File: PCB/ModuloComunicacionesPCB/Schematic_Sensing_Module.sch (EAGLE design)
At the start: 63 parts, among them IC1 MCP3202P, Q1 CSM-7X-DU, SW2 1825910-6, U1 ATMEGA328P-PU, U2 LP38690DT-5.0, U2_VCC NCP699SN33T1G, U3_VDD NCP699SN33T1G

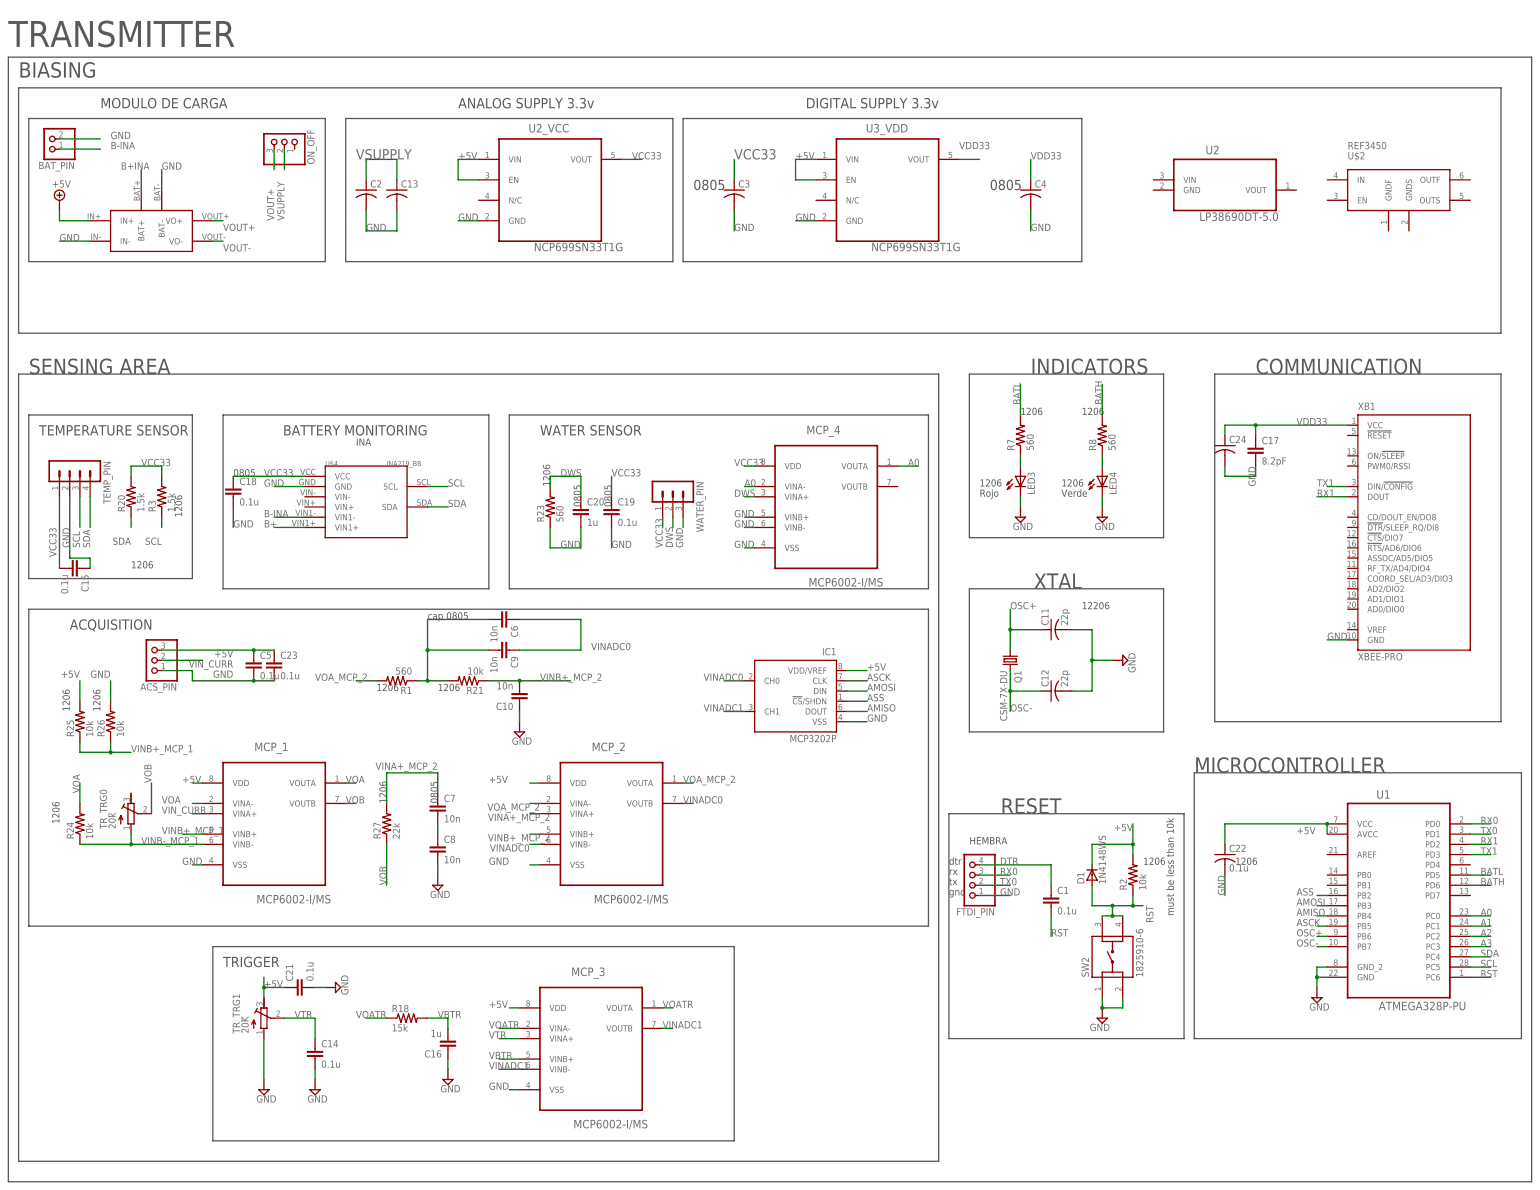
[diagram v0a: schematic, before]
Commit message: avance en esquematico para la PCB
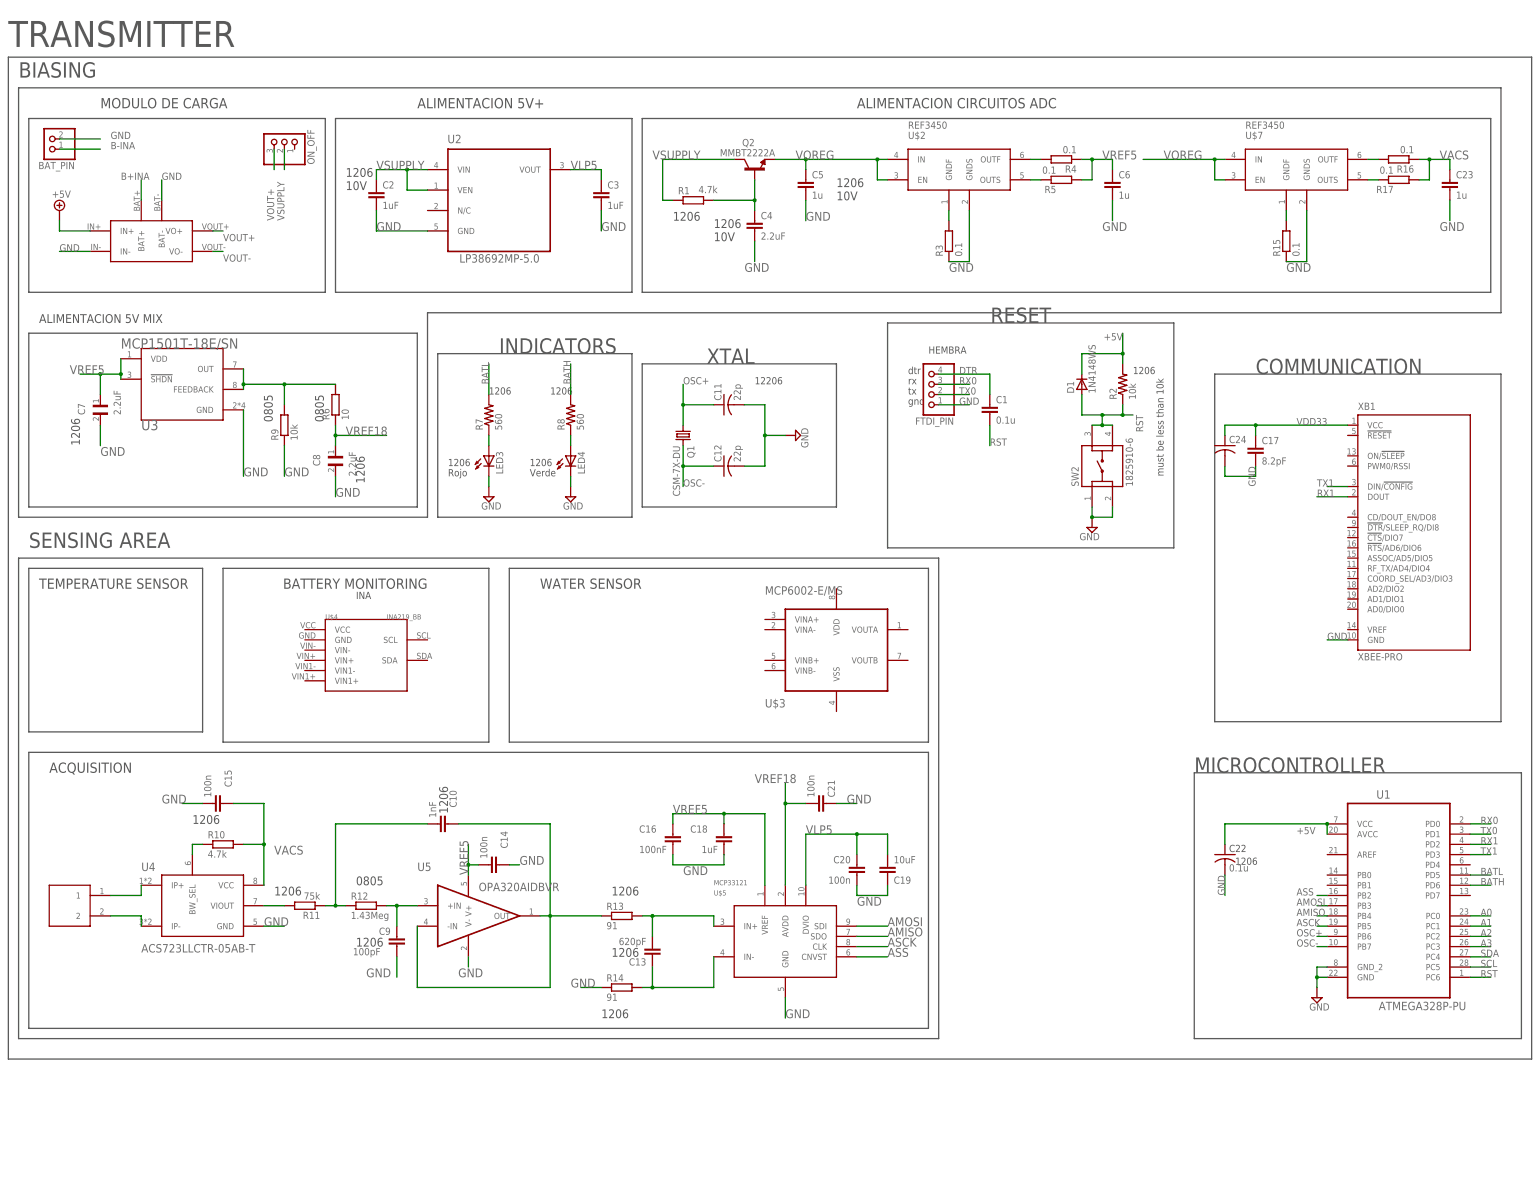
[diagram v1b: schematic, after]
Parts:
- removed ACS_PIN: (no value), pinhead:PINHD-1X3
- removed IC1: MCP3202P, microchip:MCP3202P
- removed MCP_1: MCP6002-I/MS, MCP6002-I_MS-2:MCP6002-I/MS
- removed MCP_2, MCP_3, MCP_4: MCP6002-I/MS, MCP6002-I_MS:MCP6002-I/MS
- removed R18: 15k, resistor:R-US_R0805
- removed R20: 1.5k, rcl:R-US_R1206
- removed R21, R24, R25, R26: 10k, rcl:R-US_R1206
- removed R23: 560, rcl:R-US_R1206
- removed R27: 22k, rcl:R-US_R1206
- removed TEMP_PIN: (no value), con-lstb:MA04-1
- removed TR_TRG0: 20k, rcl:R-TRIMM64W
- removed TR_TRG1: 20K, rcl:R-TRIMM64W
- removed U2_VCC, U3_VDD: NCP699SN33T1G, NCP699SN33T1G:NCP699SN33T1G
- removed WATER_PIN: (no value), con-lstb:MA03-1
- added Q2: MMBT2222A, MMBT2222A:MMBT2222A
- added R10: 4.7k, rcl:R-EU_M1206
- added R11: 75k, rcl:R-EU_R1206
- added R12: 1.43Meg, rcl:R-EU_R0805
- added R13, R14: 91, rcl:R-EU_R1206
- added R15, R16, R17, R4, R5: 0.1, rcl:R-EU_R1206
- added R6: 10, rcl:R-EU_R0805
- added R9: 10k, rcl:R-EU_R0805
- added U$3: MCP6002-E/MS, MCP6002-E_MS:MCP6002-E/MS
- added U$5: MCP33121, mcp33121:MCP33121
- added U$6: TERMINAL-TB2, TERMINAL-TB001:TERMINAL-TB2
- added U$7: REF3450, SOT95P280X145-6N:REF3450
- added U3: MCP1501T-18E/SN, MCP1501T-18E_SN:MCP1501T-18E/SN
- added U4: ACS723LLCTR-05AB-T, ACS723LLCTR-05AB-T:ACS723LLCTR-05AB-T
- added U5: OPA320AIDBVR, OPA320AIDBVR:OPA320AIDBVR
- C10: value 10n -> 1nF; device rcl:C-EUC0805 -> rcl:C-EUC1206
- C13: value (none) -> 620pF; device rcl:C-USC0805 -> rcl:C-EUC1206
- C14, C15, C21: value 0.1u -> 100n; device rcl:C-EUC0805 -> rcl:C-EUC1206
- C16: value 1u -> 100nF; device rcl:C-EUC0805 -> rcl:C-EUC1206
- C18: value 0.1u -> 1uF; device rcl:C-EUC0805 -> rcl:C-EUC1206
- C19: value 0.1u -> 10uF; device rcl:C-EUC0805 -> rcl:C-EUC1206
- C2, C3: value (none) -> 1uF; device rcl:C-USC0805 -> rcl:C-EUC1206
- C20: value 1u -> 100n; device rcl:C-EUC0805 -> rcl:C-EUC1206
- C23, C5: value 0.1u -> 1u; device rcl:C-EUC0805 -> rcl:C-EUC1206
- C4: value (none) -> 2.2uF; device rcl:C-USC0805 -> rcl:C-EUC1206
- C6: value 10n -> 1u; device rcl:C-EUC0805 -> rcl:C-EUC1206
- C7, C8: value 10n -> 2.2uF; device rcl:C-EUC0805 -> T491A106K010AT7280:T491A106K010AT7280
- C9: value 10n -> 100pF; device rcl:C-EUC0805 -> rcl:C-EUC1206
- R1: value 560 -> 4.7k; device rcl:R-US_R1206 -> rcl:R-EU_R1206
- R3: value 1.5k -> 0.1; device rcl:R-US_R1206 -> rcl:R-EU_R1206
- U2: value LP38690DT-5.0 -> LP38692MP-5.0; device LP38690DT-5.0:LP38690DT-5.0 -> LP38692MP-5.0:LP38692MP-5.0
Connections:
- removed net B+: U$4.VIN1+
- removed net DWS: C20.1, MCP_4.VINA+, R23.2, WATER_PIN.2
- removed net VBTR: C16.2, MCP_3.VINB+, R18.2
- removed net VCC33: C15.2, C18.1, C19.1, C3.1, MCP_4.VDD, R20.2, R3.2, TEMP_PIN.1, U$4.VCC, U2_VCC.VOUT, WATER_PIN.1
- removed net VINA+_MCP_2: C7.1, MCP_2.VINA+, R27.2
- removed net VINADC0: C6.1, C9.1, IC1.CH0, MCP_2.VINB-, MCP_2.VOUTB
- removed net VINADC1: IC1.CH1, MCP_3.VINB-, MCP_3.VOUTB
- removed net VINB+_MCP_1: MCP_1.VINB+, R25.1, R26.1
- removed net VINB+_MCP_2: C10.2, MCP_2.VINB+, R21.1
- removed net VINB-_MCP_1: MCP_1.VINB-, R24.1, TR_TRG0.A
- removed net VIN_CURR: ACS_PIN.2, MCP_1.VINA+
- removed net VOA: MCP_1.VINA-, MCP_1.VOUTA, R24.2
- removed net VOATR: MCP_3.VINA-, MCP_3.VOUTA, R18.1
- removed net VOA_MCP_2: MCP_2.VINA-, MCP_2.VOUTA, R1.2
- removed net VOB: MCP_1.VOUTB, R27.1, TR_TRG0.S
- removed net VTR: C14.1, MCP_3.VINA+, TR_TRG1.S
- new net N$1: R3.2, U$2.GNDF
- new net N$10: U$6.1, U4.IP+
- new net N$11: U$6.2, U4.IP-
- new net N$12: R11.2, U4.VIOUT
- new net N$14: C10.2, R11.1, R12.1
- new net N$15: C10.1, R13.1, U5.-IN, U5.OUT
- new net N$16: C13.2, R13.2, U$5.IN+
- new net N$17: C13.1, R14.2, U$5.IN-
- new net N$18: R16.2, U$7.OUTF
- new net N$19: R17.2, U$7.OUTS
- new net N$2: C4.1, Q2.B, R1.2
- new net N$20: R15.2, U$7.GNDF
- new net N$6: R5.2, U$2.OUTS
- new net N$7: R6.2, R9.2, U3.FEEDBACK, U3.OUT
- new net N$8: R10.1, U4.BW_SEL
- new net VACS: C15.1, C23.1, R10.2, R16.1, R17.1, U4.VCC
- new net VLP5: C19.2, C20.1, C3.1, U$5.DVIO, U2.VOUT
- new net VOREG: C5.1, Q2.E, U$2.EN, U$2.IN, U$7.EN, U$7.IN
- new net VREF18: C21.2, C8.1, R6.1, U$5.AVDD
- new net VREF5: C14.2, C16.1, C18.1, C6.1, C7.1, R4.1, R5.1, U$5.VREF, U3.!SHDN, U3.VDD, U5.V+
- net +5V: no longer ACS_PIN.3, C21.1, C23.1, C5.1, IC1.VDD/VREF, MCP_1.VDD, MCP_2.VDD, MCP_3.VDD, R25.2, TR_TRG1.E, U2_VCC.EN, U2_VCC.VIN, U3_VDD.EN, U3_VDD.VIN
- net A0: no longer MCP_4.VINA-, MCP_4.VOUTA
- net AMISO: now also U$5.SDO; no longer IC1.DOUT
- net AMOSI: now also U$5.SDI; no longer IC1.DIN
- net ASCK: now also U$5.CLK; no longer IC1.CLK
- net ASS: now also U$5.CNVST; no longer IC1.!CS!/SHDN
- net B-INA: no longer U$4.VIN1-
- net GND: now also C14.1, C15.2, C16.2, C19.1, C21.1, C6.2, C7.2, C9.2, R14.1, R15.1, R3.1, R9.1, U$2.GNDS, U$5.GND, U$7.GNDS, U2.GND, U3.GND, U4.GND, U5.V-; no longer ACS_PIN.1, C10.1, C13.2, C14.2, C15.1, C16.1, C19.2, C21.2, IC1.VSS, MCP_1.VSS, MCP_2.VSS, MCP_3.VSS, MCP_4.VINB+, MCP_4.VINB-, MCP_4.VSS, R23.1, R26.2, TEMP_PIN.2, TR_TRG1.A, U$4.GND, U2_VCC.GND, U3_VDD.GND, WATER_PIN.3
- net N$13: now also C9.1, R12.2, U5.+IN; no longer C6.2, C9.2, R1.1, R21.2
- net N$5: now also R4.2, U$2.OUTF; no longer C7.2, C8.1
- net SCL: no longer R3.1, TEMP_PIN.3, U$4.SCL
- net SDA: no longer R20.1, TEMP_PIN.4, U$4.SDA
- net VDD33: no longer C4.1, U3_VDD.VOUT
- net VSUPPLY: now also Q2.C, R1.1, U2.VEN, U2.VIN; no longer C13.1
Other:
- note added: "1206 10V"
- note added: "ALIMENTACION 5V MIX"
- note added: "ALIMENTACION 5V+"
- note added: "ALIMENTACION CIRCUITOS ADC"
- note removed: "ANALOG SUPPLY 3.3v"
- note removed: "DIGITAL SUPPLY 3.3v"
- note removed: "TRIGGER"
- note removed: "cap 0805"
- moved on the sheet: C1, C10, C11, C12, C13, C14, C15, C16, C18, C19, C2, C20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
